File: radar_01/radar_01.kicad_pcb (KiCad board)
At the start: 2 copper layers, 77.5 x 44.5 mm, 45 parts, among them J1 Power, J2 Out, M1 dcdc5v, U1 LM358, U2 HB-100-Radar, U3 LM2903

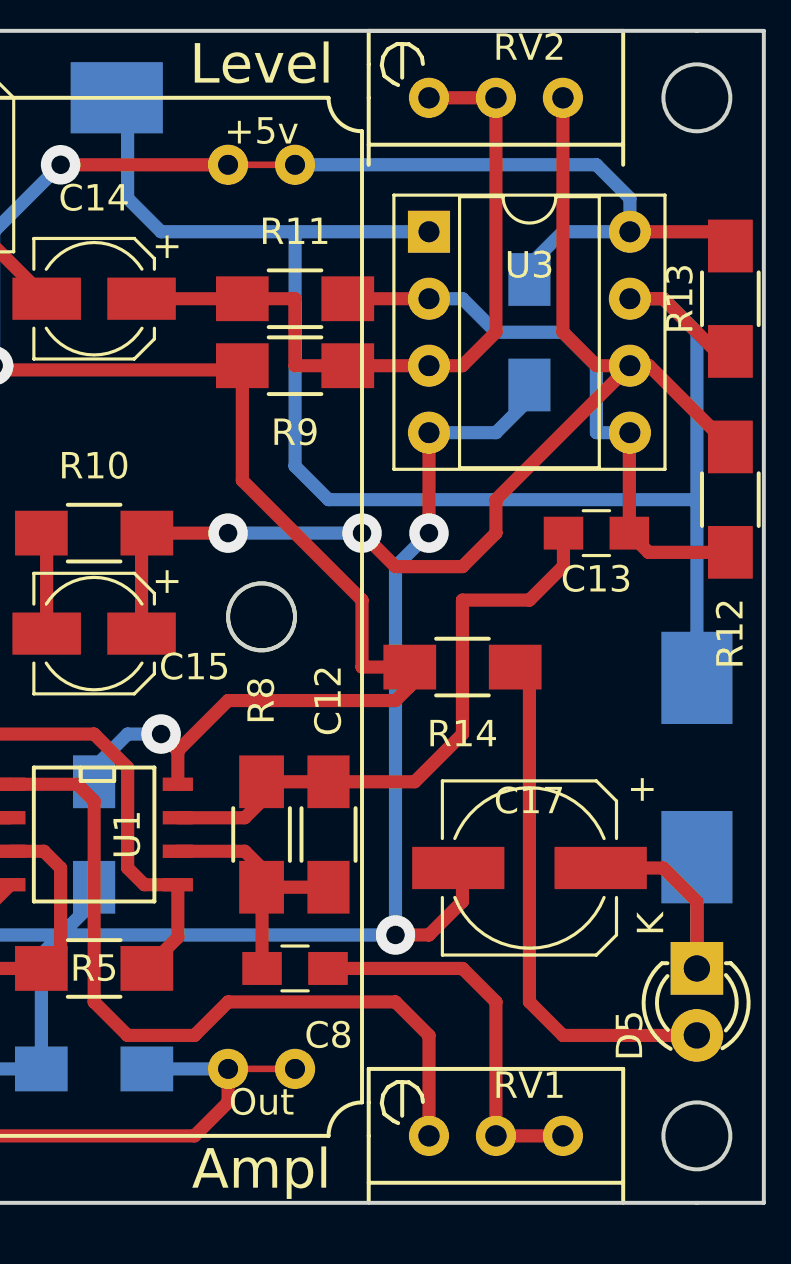
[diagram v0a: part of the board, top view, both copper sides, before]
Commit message: update
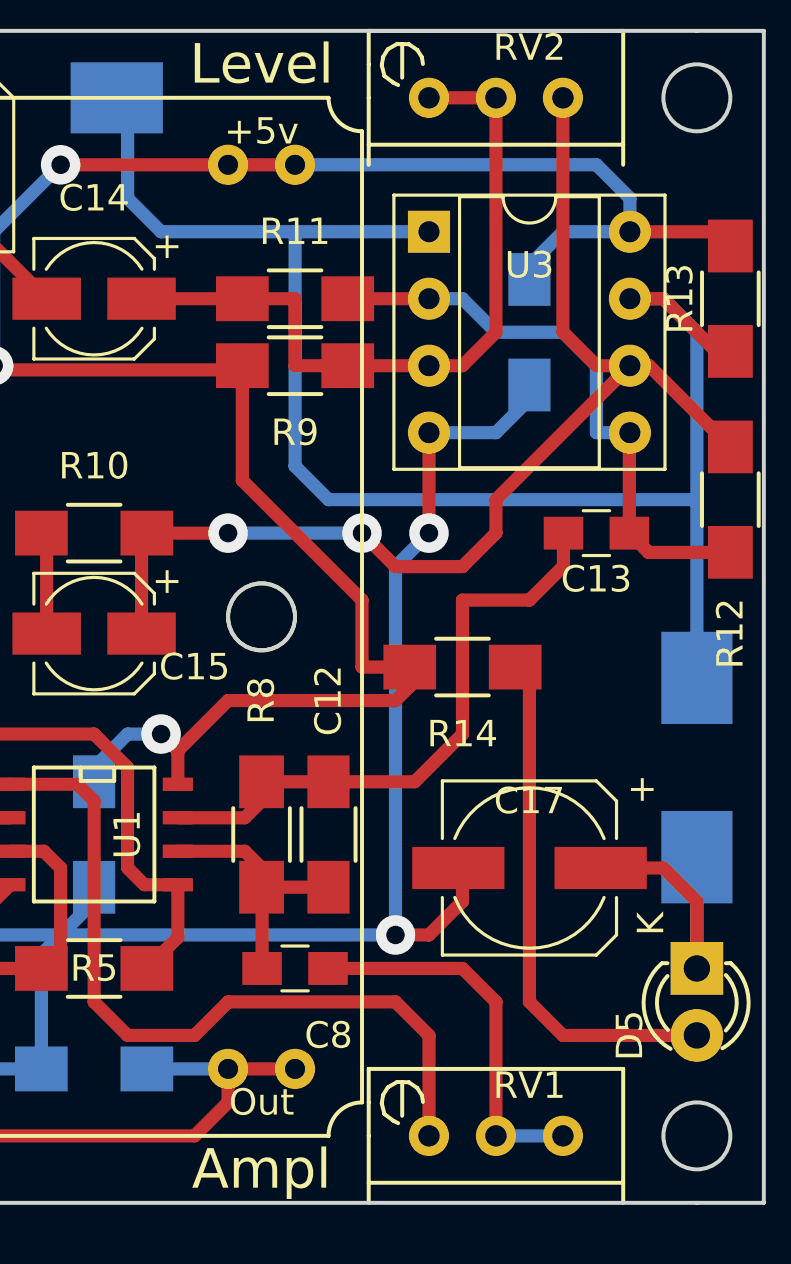
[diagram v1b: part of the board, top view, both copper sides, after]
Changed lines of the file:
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@@
   (segment (start 202.565 85.725) (end 203.2 86.36) (width 0.5) (layer F.Cu) (net 1))
   (segment (start 203.2 89.44) (end 202.47 90.17) (width 0.5) (layer F.Cu) (net 1) (status 30))
-  (segment (start 209.55 93.98) (end 212.09 93.98) (width 0.25) (layer F.Cu) (net 2))
+  (segment (start 209.55 93.98) (end 212.09 93.98) (width 0.5) (layer F.Cu) (net 2))
   (segment (start 206.47 93.98) (end 209.55 93.98) (width 0.5) (layer B.Cu) (net 2) (status 30))
   (segment (start 196.85 94.51) (end 196.85 95.25) (width 0.5) (layer F.Cu) (net 2) (status 30))
@@
   (segment (start 200.025 84.455) (end 197.39 87.09) (width 0.5) (layer F.Cu) (net 6) (status 20))
   (segment (start 197.39 87.09) (end 196.85 87.09) (width 0.5) (layer F.Cu) (net 6) (status 30))
+  (segment (start 209.55 59.69) (end 212.09 59.69) (width 0.5) (layer F.Cu) (net 7))
   (segment (start 224.79 62.23) (end 228.06 62.23) (width 0.5) (layer F.Cu) (net 7))
   (segment (start 228.06 62.23) (end 228.6 62.77) (width 0.5) (layer F.Cu) (net 7))
@@
   (segment (start 216.44 79.47) (end 215.9 80.01) (width 0.5) (layer F.Cu) (net 7))
   (segment (start 215.9 80.01) (end 209.55 80.01) (width 0.5) (layer F.Cu) (net 7))
-  (segment (start 209.55 59.69) (end 212.09 59.69) (width 0.25) (layer F.Cu) (net 7))
   (segment (start 168.29 68.47) (end 165.79 68.47) (width 0.5) (layer B.Cu) (net 7))
   (segment (start 165.79 68.47) (end 165.68 68.58) (width 0.5) (layer B.Cu) (net 7))
@@
   (segment (start 210.185 85.725) (end 210.82 86.36) (width 0.5) (layer F.Cu) (net 9) (status 20))
   (segment (start 210.82 86.36) (end 210.82 87.09) (width 0.5) (layer F.Cu) (net 9) (status 30))
-  (segment (start 219.71 96.52) (end 222.25 96.52) (width 0.5) (layer F.Cu) (net 10) (status 30))
+  (segment (start 219.71 96.52) (end 222.25 96.52) (width 0.5) (layer B.Cu) (net 10))
   (segment (start 219.71 96.52) (end 219.71 91.44) (width 0.5) (layer F.Cu) (net 10) (status 10))
   (segment (start 219.71 91.44) (end 218.44 90.17) (width 0.5) (layer F.Cu) (net 10))
